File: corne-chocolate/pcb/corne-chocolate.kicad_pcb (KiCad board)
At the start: 2 copper layers, 133.8 x 91.4 mm, 98 parts, among them J3 LED, P1 i2c-pin, P2 i2c-pin, SW1 SW_PUSH, SW10 SW_PUSH, SW11 SW_PUSH, SW12 SW_PUSH, SW13 SW_PUSH, SW14 SW_PUSH, SW15 SW_PUSH, SW16 SW_PUSH, SW17 SW_PUSH, SW18 SW_PUSH, SW19 SW_PUSH, SW2 SW_PUSH, SW20 SW_PUSH, SW21 SW_PUSH, SW3 SW_PUSH, SW4 SW_PUSH, SW5 SW_PUSH, SW6 SW_PUSH, SW7 SW_PUSH, SW8 SW_PUSH, SW9 SW_PUSH, U1 ProMicro

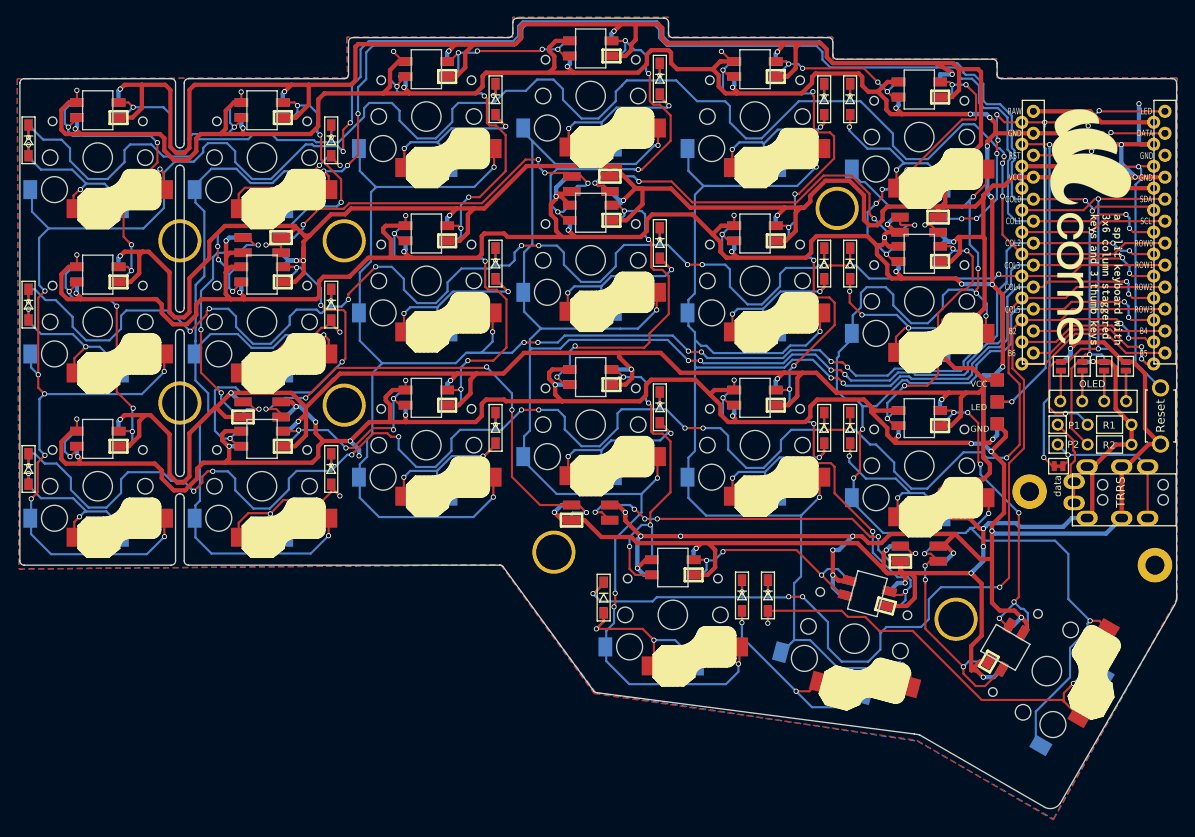
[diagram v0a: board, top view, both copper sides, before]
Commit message: saving using kicad 6
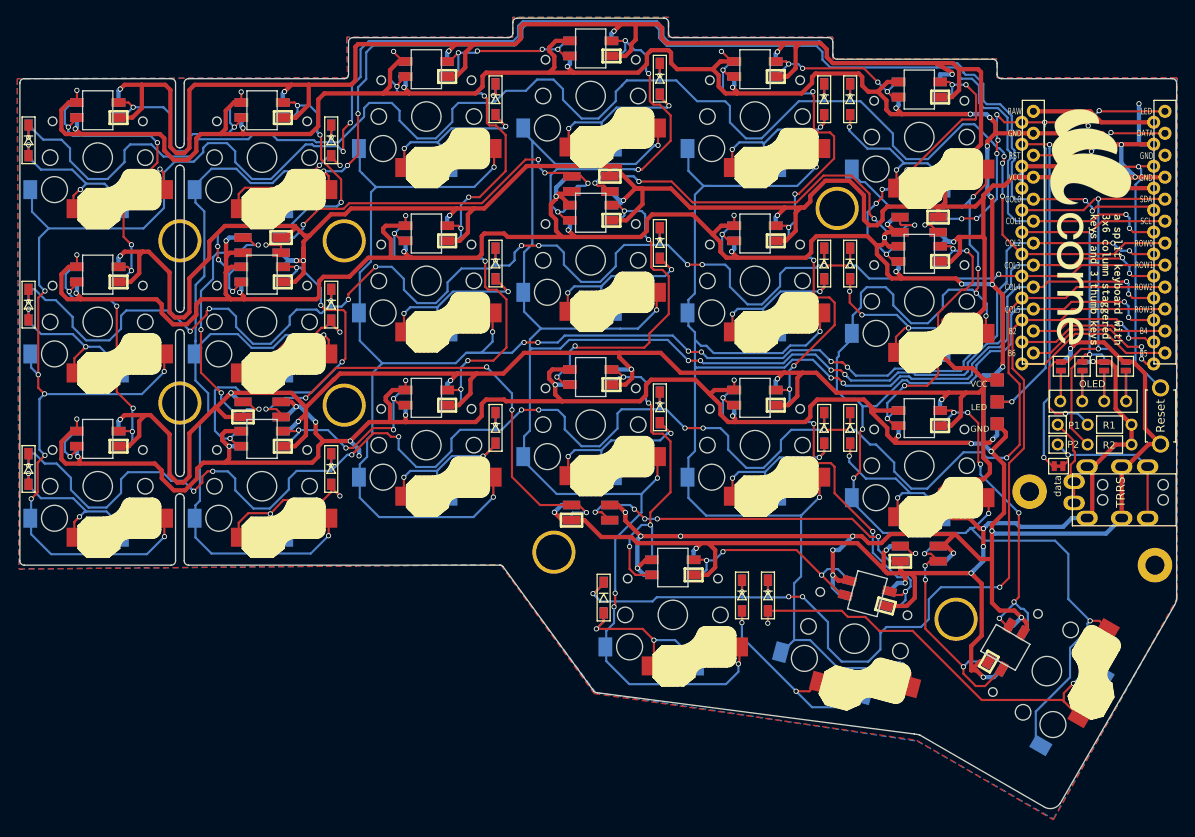
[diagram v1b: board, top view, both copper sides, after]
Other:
- net class Default removed
